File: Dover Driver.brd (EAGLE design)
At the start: 62.2 x 62.2 mm, 44 parts

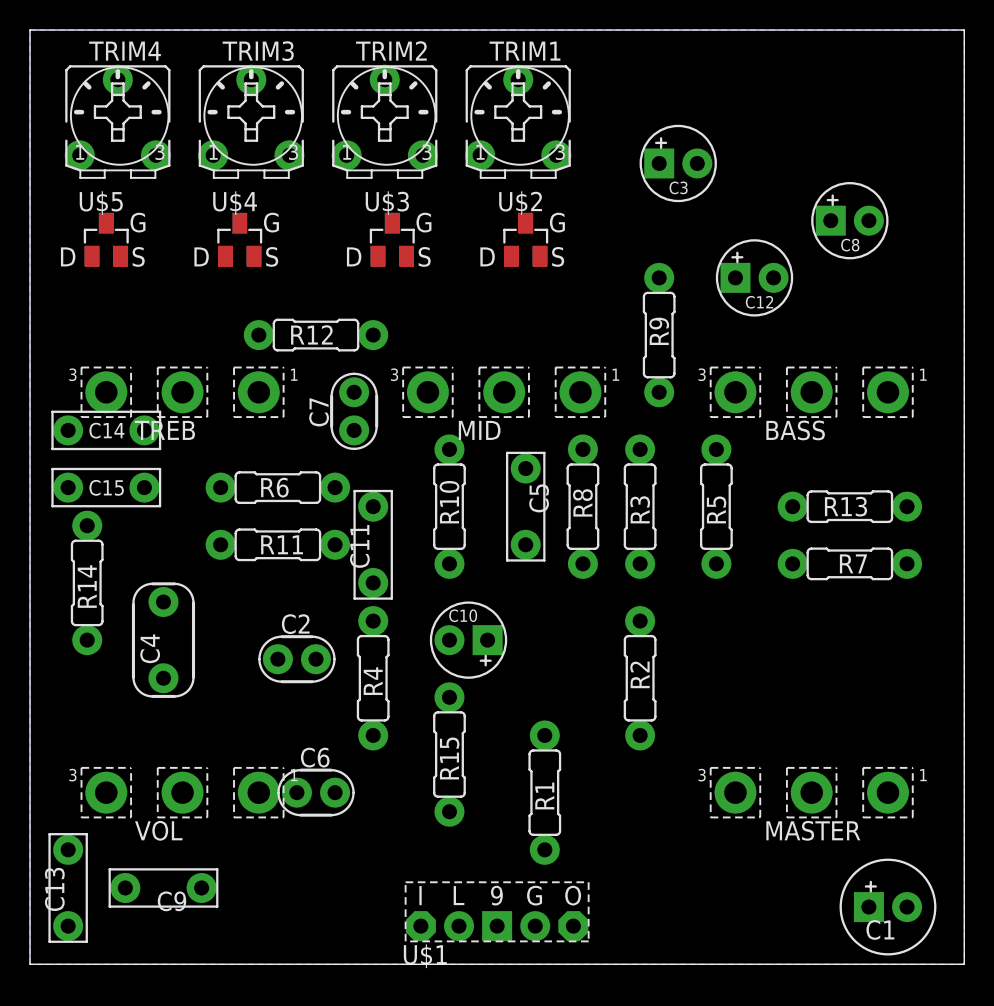
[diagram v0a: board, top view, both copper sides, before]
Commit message: Version 1.0 layout finished
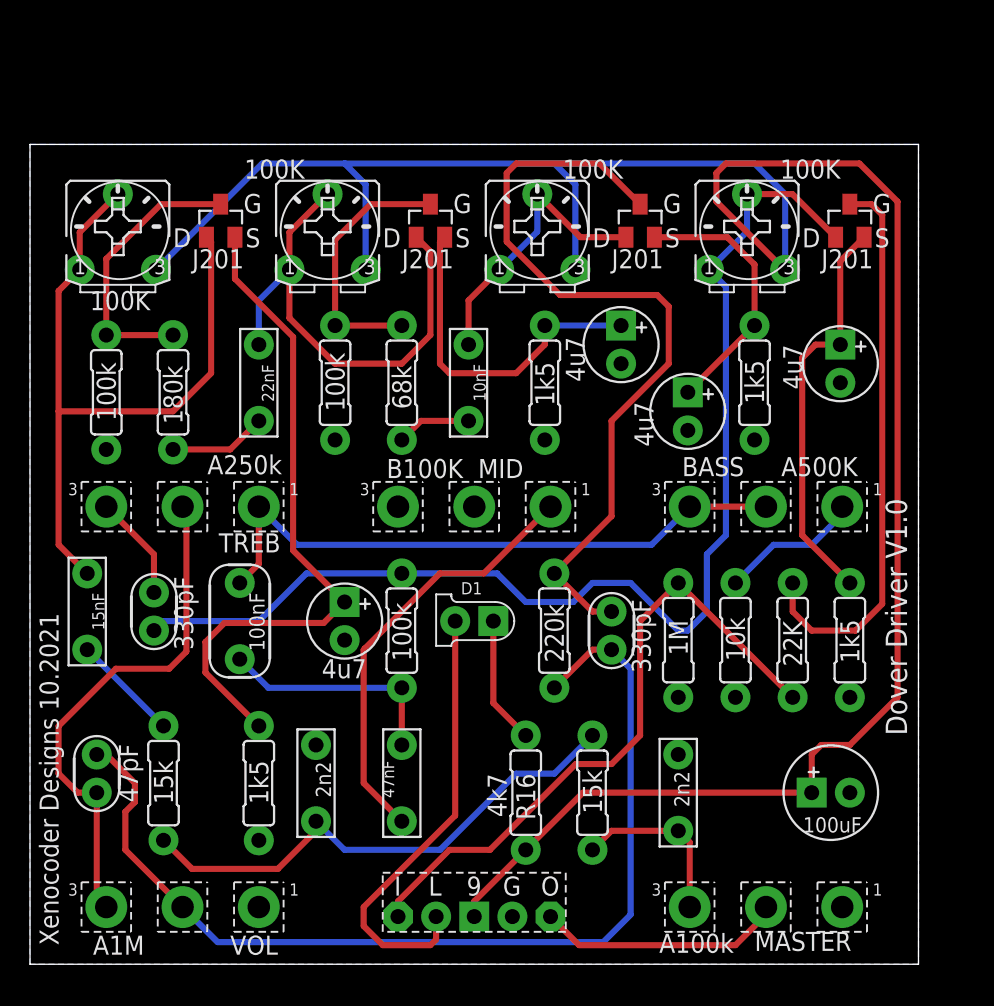
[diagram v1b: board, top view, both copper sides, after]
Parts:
- added D1: LED3MM, mb_diodes:LED3MM
- added R16: 4k7, mb_resistors:R0207/3
- C10, C12, C3, C8: value 4k7 -> 4u7
- U$2: value MMBFj201 -> J201
- U$3, U$4, U$5: value MMBFJ201 -> J201
- moved R13 43.5 mm to (15.2, 12.1), turned to 90 degrees
- moved C15 43.2 mm to (43.2, 11.4), turned to 90 degrees
- moved C9 39.3 mm to (29.2, 38.7), turned to 90 degrees
- moved C12 35.6 mm to (21.0, 22.9), turned to 270 degrees
- moved C14 27.3 mm to (19.1, 12.1), turned to 90 degrees
- moved C7 22.5 mm to (38.7, 22.2)
- moved C10 22.2 mm to (39.4, 41.3), turned to 270 degrees
- moved R9 21.8 mm to (20.3, 38.7), turned to 90 degrees
- moved U$2 21.6 mm to (54.6, 49.5)
- moved R6 20.7 mm to (34.9, 22.2), turned to 270 degrees
- moved C5 20.2 mm to (24.8, 12.1), turned to 90 degrees
- moved C13 18.5 mm to (3.81, 23.5)
- moved C3 17.2 mm to (54.0, 40.0), turned to 270 degrees
- moved TRIM1 17.0 mm to (48.3, 48.3)
- moved C8 16.7 mm to (43.8, 36.8), turned to 270 degrees
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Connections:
- new net N$28: D1.A, R16.1
- new net N$29: D1.K, U$1.2
- net N$5: now also R16.2
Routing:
- net N$5: track 0.00 -> 157.1 mm
- net N$4: track 0.00 -> 78.5 mm
- net N$12: track 0.00 -> 68.0 mm
- net N$13: track 0.00 -> 53.2 mm
- net N$23: track 0.00 -> 48.1 mm
- net N$22: track 0.00 -> 44.8 mm
- net N$1: track 0.00 -> 43.7 mm
- net N$9: track 0.00 -> 41.5 mm
- net N$2: track 0.00 -> 37.5 mm
- net N$25: track 0.00 -> 35.0 mm
- net N$11: track 0.00 -> 34.4 mm
- net N$18: track 0.00 -> 33.5 mm
- net N$29: track 0.00 -> 29.9 mm
- net N$8: track 0.00 -> 28.9 mm
- net N$3: track 0.00 -> 27.0 mm
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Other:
- board size 62.2 x 62.2 mm -> 59.2 x 54.6 mm
- board text added: "Dover Driver V1.0"
- board text added: "Xenocoder Designs 10.2021"
